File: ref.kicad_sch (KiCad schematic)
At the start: 44 parts, among them Q1 Q_NPN_BCE, U4 ADR1000, U5 Opamp_Dual, U8 ADA4523-1

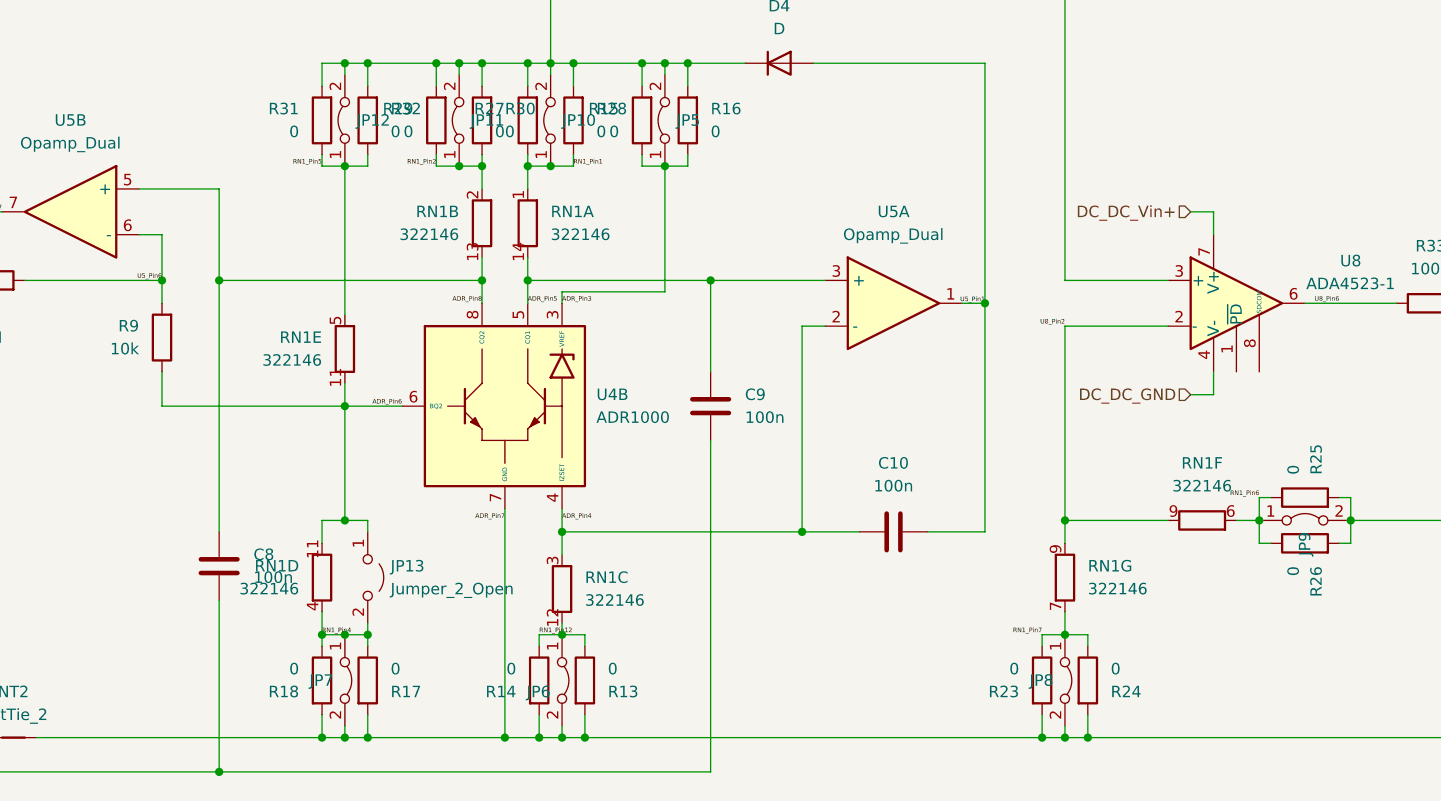
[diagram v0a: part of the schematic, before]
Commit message: asdf
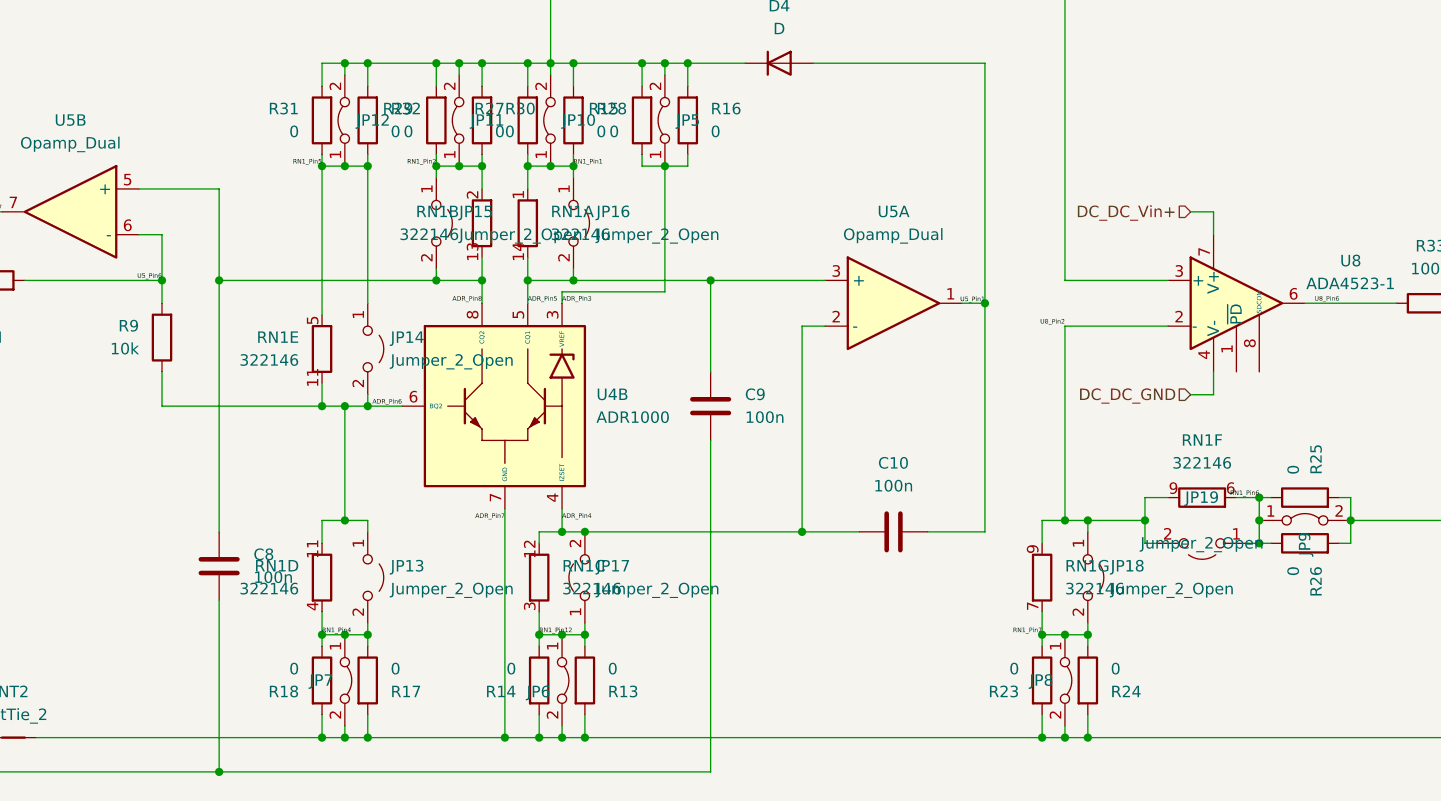
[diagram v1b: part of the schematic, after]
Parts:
- added JP14, JP15, JP16, JP17, JP18, JP19: Jumper_2_Open, Jumper:SolderJumper-2_P1.3mm_Open_RoundedPad1.0x1.5mm, symbol Jumper:Jumper_2_Open
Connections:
- net ADR_Pin4: now also RN1.12 (R3.2), JP17.2 (B); no longer RN1.3 (R3.1)
- net ADR_Pin5: now also JP16.2 (B)
- net ADR_Pin6: now also JP14.2 (B)
- net ADR_Pin8: now also JP15.2 (B)
- net RN1_Pin1: now also JP16.1 (A)
- net RN1_Pin12: now also RN1.3 (R3.1), JP17.1 (A); no longer RN1.12 (R3.2)
- net RN1_Pin2: now also JP15.1 (A)
- net RN1_Pin5: now also JP14.1 (A)
- net RN1_Pin6: now also JP19.1 (A)
- net RN1_Pin7: now also JP18.2 (B)
- net U8_Pin2: now also JP18.1 (A), JP19.2 (B)
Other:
- moved on the sheet: RN1C, RN1E, RN1F, RN1G
